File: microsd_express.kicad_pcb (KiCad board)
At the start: 2 copper layers, 26.7 x 16.8 mm, 25 parts, among them J1 10102166A812A, J2 Conn_01x16, U1 MIC2230-GSYML-TR

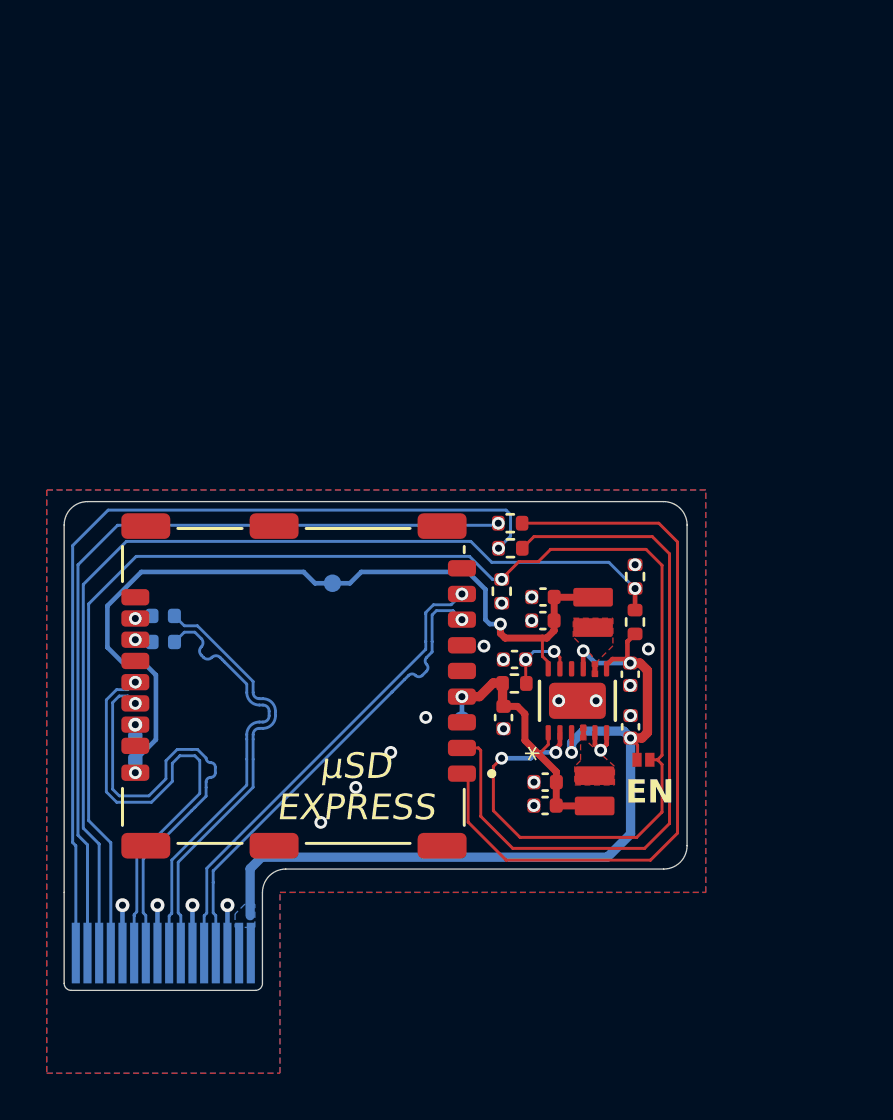
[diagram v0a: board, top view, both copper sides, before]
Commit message: Initial Commit to Fork
Design is mostly completed, still requires layout
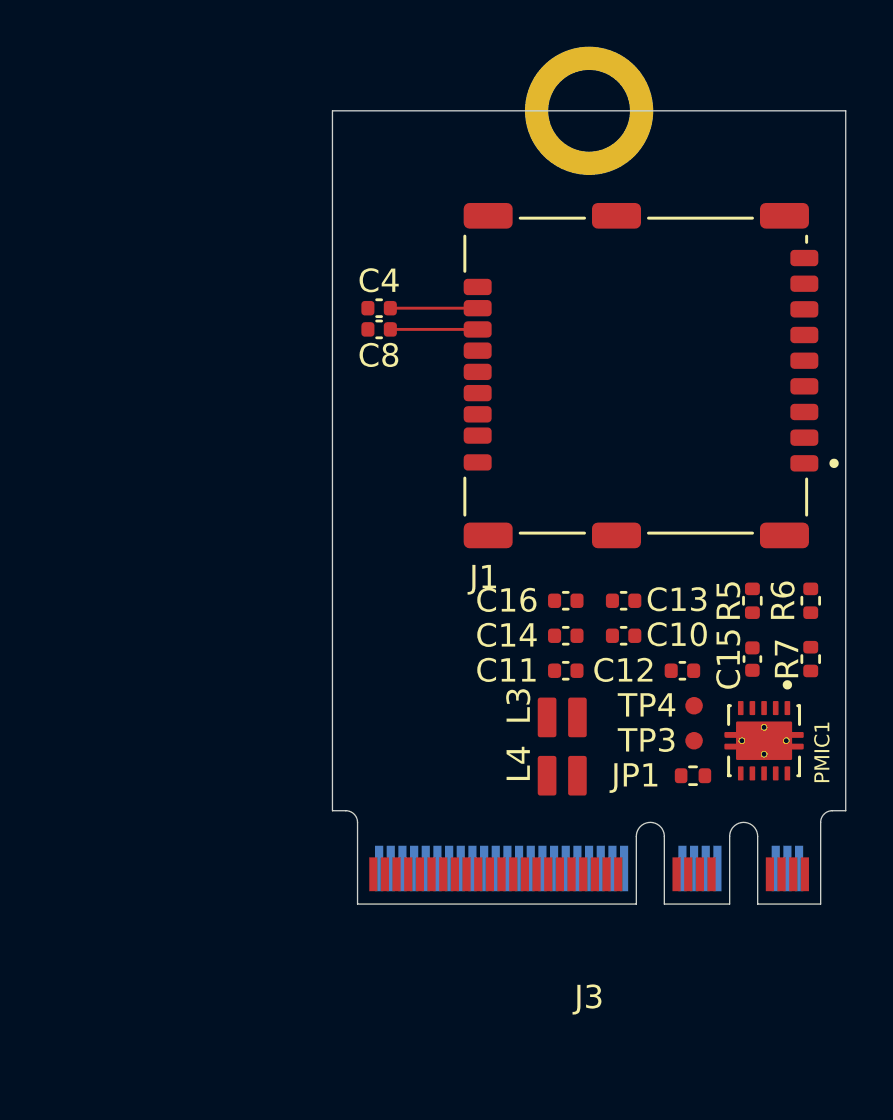
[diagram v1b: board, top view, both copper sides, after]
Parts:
- removed C1, C2, C3, C5, C6, C7: 22u, Capacitor_SMD:C_0402_1005Metric
- removed C9: 220n, Capacitor_SMD:C_0402_1005Metric
- removed J2: Conn_01x16, 1Library:PCIe_connector
- removed L1, L2: 2.2u, 1Library:F1C1-201612-2R2M
- removed R1: 33, Resistor_SMD:R_0402_1005Metric
- removed R2: 100k, Resistor_SMD:R_0402_1005Metric
- removed R3: 3k6, Resistor_SMD:R_0402_1005Metric
- removed R4: 6k8, Resistor_SMD:R_0402_1005Metric
- removed TP1, TP2: TestPoint, 1Library:testpoint
- removed U1: MIC2230-GSYML-TR, 1Library:MLF-12_YML_MCH-L
- added ?: , M.2-Templates:M.2-KEY-BLANK, F.Cu at (126.0, 45.0)
- added C12: 10u, Capacitor_SMD:C_0402_1005Metric, F.Cu at (130.0, 69.0)
- added C13: 22u, Capacitor_SMD:C_0402_1005Metric, F.Cu at (127.5, 66.0)
- added C14: 22u, Capacitor_SMD:C_0402_1005Metric, F.Cu at (125.0, 67.5)
- added C15: 22u, Capacitor_SMD:C_0402_1005Metric, F.Cu at (133.0, 68.5)
- added C16: 22u, Capacitor_SMD:C_0402_1005Metric, F.Cu at (125.0, 66.0)
- added J3: Conn_2Rows-75Pins, NGFF:NGFF_A+E, F.Cu at (126.0, 79.0)
- added L3: 2.2u, 1Library:F1C1-201612-2R2M, F.Cu at (124.8, 71.0)
- added L4: 2.2u, 1Library:F1C1-201612-2R2M, F.Cu at (124.8, 73.5)
- added PMIC1: ~, TPS62402QDRCRQ1:SON50P300X300X100-11N, F.Cu at (133.5, 72.0)
- added R7: 33, Resistor_SMD:R_0402_1005Metric, F.Cu at (135.5, 68.5)
- added TP3: TestPoint, 1Library:testpoint, F.Cu at (130.5, 72.0)
- added TP4: TestPoint, 1Library:testpoint, F.Cu at (130.5, 70.5)
- C10, C4, C8: moved to F.Cu
- JP1: value Jumper_2_Open -> Jumper; footprint 1Library:Jumper -> Resistor_SMD:R_0402_1005Metric
- moved C10 21.5 mm to (127.5, 67.5), turned to 0 degrees
- moved J1 19.8 mm to (128.0, 56.4)
- moved C8 16.3 mm to (117.0, 54.4), turned to 0 degrees
- moved C4 16.1 mm to (117.0, 53.5), turned to 0 degrees
- moved R6 13.3 mm to (135.5, 66.0), turned to 90 degrees
- moved R5 10.6 mm to (133.0, 66.0), turned to 90 degrees
- moved C11 3.34 mm to (125.0, 69.0), turned to 0 degrees
- moved JP1 2.00 mm to (130.5, 73.5), turned to 0 degrees
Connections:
- net Net-(C4-Pad2) renamed /PCIE_RX_P_CARD
- net Net-(C8-Pad2) renamed /PCIE_RX_N_CARD
- JP1 pad 1: /PCIE_PWR_EN -> /PCIE_VIN
- JP1 pad 2: +5V -> /NET_VIN
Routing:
- net /PCIE_PWR_EN: track 66.4 -> 0.00 mm, vias 3 -> 0
- net /PCIE_DET_WAKE: track 41.7 -> 0.00 mm, vias 1 -> 0
- net +5V: track 38.4 -> 0.00 mm, vias 4 -> 0
- net /PCIE_RST_B: track 38.1 -> 0.00 mm, vias 1 -> 0
- net +1V8: track 35.9 -> 0.00 mm, vias 2 -> 0
- net /PCIE_CLKREQ_N: track 35.0 -> 0.00 mm, vias 1 -> 0
- net /PCIE_CLKREQ_N_CARD: track 31.8 -> 0.00 mm
- net /PCIE_RST_B_CARD: track 31.2 -> 0.00 mm
- net /PCIE_TX_N: track 19.9 -> 0.00 mm, vias 1 -> 0
- net /PCIE_TX_P: track 19.8 -> 0.00 mm, vias 1 -> 0
- net /PCIE_CLK_N: track 19.8 -> 0.00 mm, vias 1 -> 0
- net /PCIE_CLK_P: track 19.8 -> 0.00 mm, vias 1 -> 0
- net /PCIE_RX_P: track 18.2 -> 0.00 mm
- net /PCIE_RX_N: track 18.2 -> 0.00 mm
- net +3V3: track 12.5 -> 0.00 mm, vias 1 -> 0
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- removed copper zone on B.Cu, net +5V
- removed copper zone on B.Cu, net GND
- removed copper zone on F.Cu, net GND
- removed copper zone on F.Cu, net Net-(U1-SW1)
- removed copper zone on F.Cu, net Net-(U1-SW2)
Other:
- board size 26.7 x 16.8 mm -> 22 x 30 mm
- board text added: "TP3"
- board text added: "TP4"
- board text removed: "1v8"
- board text removed: "3v3"
- board text removed: "EN"
- board text removed: "STIFFENER 0.1MM PI TOP SIDE"
- board text removed: "µSD EXPRESS"
